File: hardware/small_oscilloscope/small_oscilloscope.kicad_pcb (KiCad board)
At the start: 2 copper layers, 181.6 x 99.1 mm, 104 parts, among them J1 Conn_01x16, J2 Conn_01x16, J3 Conn_Coaxial, J4 Conn_Coaxial, J5 Parellel LCD, J6 Conn_01x02, J7 Conn_01x03, Q1 NTR5103NT1G, Q2 NTR5103NT1G, Q3 NTR5103NT1G, Q4 NTR5103NT1G, Q5 NTR5103NT1G, Q6 NTR5103NT1G, Q7 NTR5103NT1G, Q8 NTR5103NT1G, Q9 NTR5103NT1G, SW1 SW_MEC_5E, SW2 RotaryEncoder_Switch_MP, SW3 SW_MEC_5E, SW4 SW_MEC_5E, SW5 SW_MEC_5E, SW6 RotaryEncoder_Switch_MP, U1 CH423S, U10 EA2208T6R, U11 FT800Q-T, U12 LM358, U13 L79L05_TO92, U2 TMUX1101DBV, U3 TMUX1101DBV, U4 TMUX1101DBV, U5 TMUX1101DBV, U6 TL084, U7 LM311, U8 LM311, U9 NE555P, Y1 12.0000M

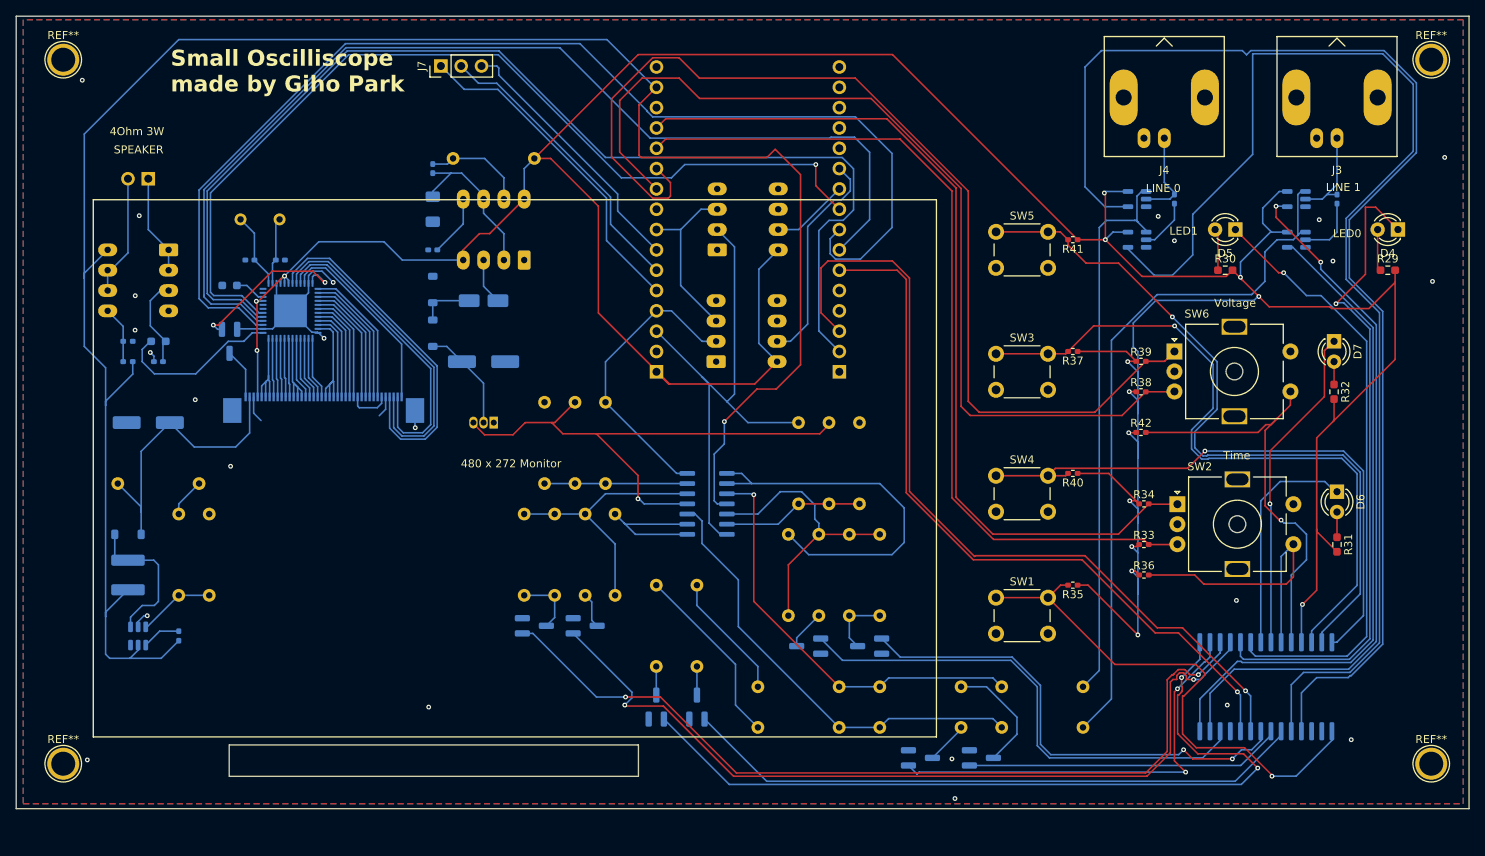
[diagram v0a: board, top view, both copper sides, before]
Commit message: oscilliscope first success
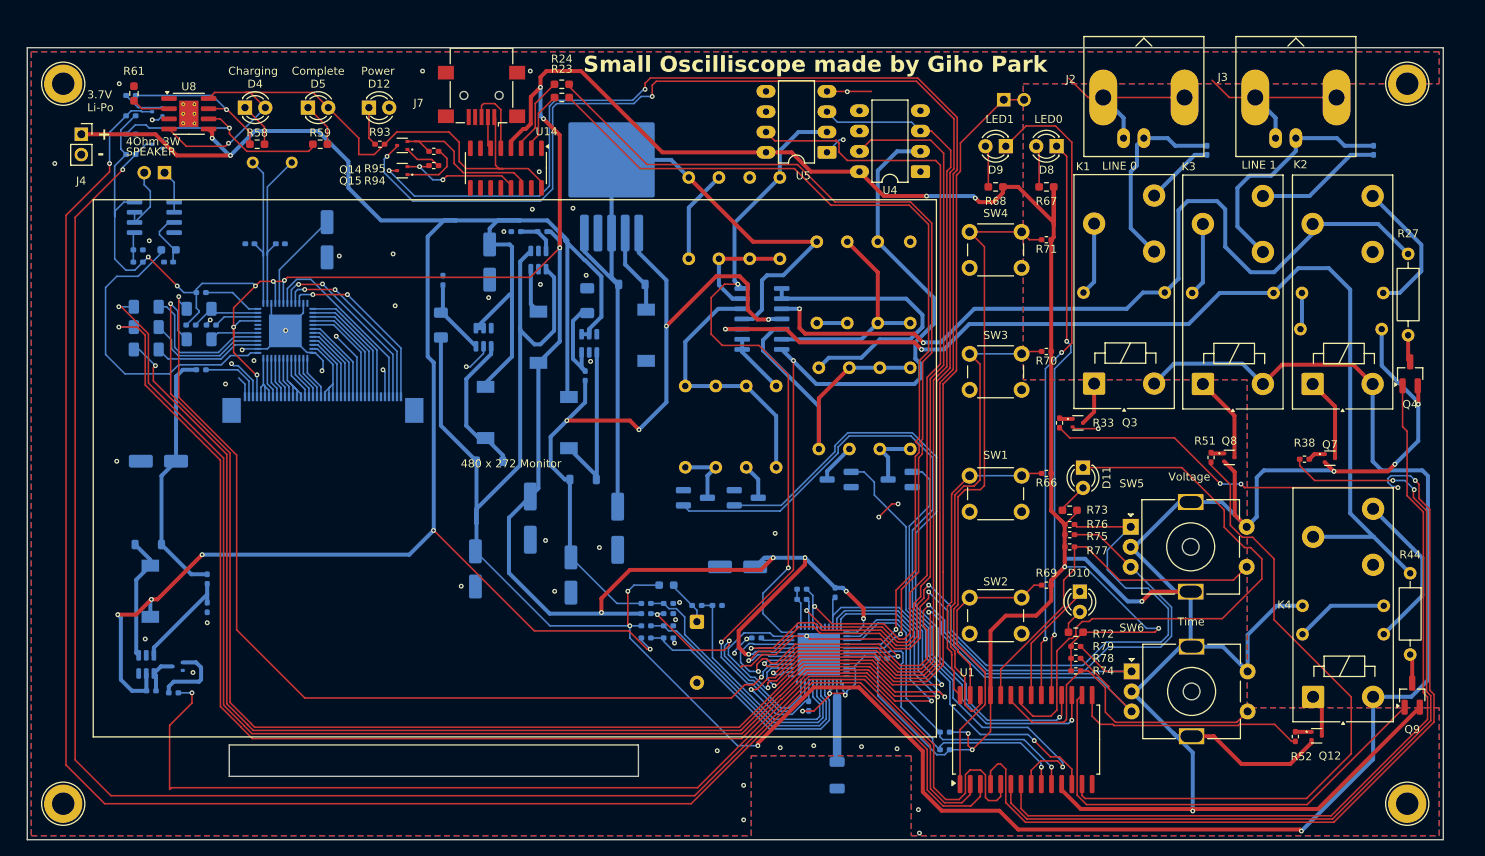
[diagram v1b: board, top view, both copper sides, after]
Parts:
- removed the C3 at (123.2, 59.7)
- removed the C4 at (123.2, 64.8)
- removed the C6 at (129.5, 78.7)
- removed the D2 at (123.2, 75.2)
- removed the J2 at (174.0, 80.0)
- removed the Q9 at (97.8, 76.2)
- removed the R25 at (123.2, 54.6)
- removed the R27 at (91.4, 97.8)
- removed the REF** at (248.0, 41.0)
- removed the REF** at (77.0, 41.0)
- removed the REF** at (77.0, 129.0)
- removed the REF** at (248.0, 129.0)
- removed the U13 at (130.8, 86.4)
- removed the U3 at (231.1, 58.4)
- removed the U4 at (211.2, 63.5)
- removed the U5 at (211.2, 58.4)
- added AE1: Antenna_Chip, Inductor_SMD:L_1206_3216Metric_Pad1.22x1.90mm_HandSolder, B.Cu at (173.7, 130.4)
- added C1: 10u, Capacitor_SMD:CP_Elec_5x5.3, B.Cu at (161.3, 104.4)
- added C10: 10u, Capacitor_SMD:CP_Elec_6.3x5.7, B.Cu at (146.3, 99.6)
- added C13: 10u, Capacitor_SMD:CP_Elec_5x5.3, B.Cu at (110.0, 63.5)
- added C2: 0.1u, Capacitor_SMD:C_0402_1005Metric_Pad0.74x0.62mm_HandSolder, B.Cu at (179.4, 115.8)
- added C7: 47u, Capacitor_SMD:CP_Elec_5x5.3, B.Cu at (140.5, 105.4)
- added C8: 100u, Capacitor_SMD:CP_Elec_5x5.3, B.Cu at (128.5, 104.6)
- added C9: 47u, Capacitor_SMD:CP_Elec_6.3x5.7, B.Cu at (135.4, 98.3)
- added D12: LED, LED_THT:LED_D3.0mm, F.Cu at (115.2, 47.0)
- added D3: 1N5819, Diode_SMD:D_SOD-123, B.Cu at (142.0, 93.5)
- added D4: LED_Small, LED_THT:LED_D3.0mm, F.Cu at (99.7, 47.0)
- added D5: LED_Small, LED_THT:LED_D3.0mm, F.Cu at (107.6, 47.0)
- added D6: 1N5819, Diode_SMD:D_SOD-123, B.Cu at (130.3, 91.2)
- added D7: 1N5819, Diode_SMD:D_SOD-123, B.Cu at (148.1, 69.1)
- added J4: BAT, Connector_PinSocket_2.54mm:PinSocket_1x02_P2.54mm_Vertical, F.Cu at (79.3, 50.3)
- added K1: FINDER-40.41, Relay_THT:Relay_SPDT_Finder_40.41, F.Cu at (205.9, 81.5)
- added K2: FINDER-40.41, Relay_THT:Relay_SPDT_Finder_40.41, F.Cu at (233.2, 81.5)
- added K3: FINDER-40.41, Relay_THT:Relay_SPDT_Finder_40.41, F.Cu at (219.5, 81.5)
- added K4: FINDER-40.41, Relay_THT:Relay_SPDT_Finder_40.41, F.Cu at (233.2, 120.6)
- added L2: 10u, Inductor_SMD:L_7.3x7.3_H3.5, B.Cu at (140.2, 86.4)
- added L3: 10u, Inductor_SMD:L_7.3x7.3_H3.5, B.Cu at (129.8, 85.1)
- added L4: 10u, Inductor_SMD:L_7.3x7.3_H3.5, B.Cu at (136.4, 75.7)
- added L5: 100u, Inductor_SMD:L_7.3x7.3_H3.5, B.Cu at (149.9, 75.4)
- added Q1: 2SC4671, Package_TO_SOT_SMD:SOT-523, B.Cu at (88.8, 47.5)
- added Q12: 2SC4671, Package_TO_SOT_SMD:SOT-523, F.Cu at (233.7, 125.5)
- added Q13: 2SC4671, Package_TO_SOT_SMD:SOT-523, B.Cu at (91.3, 116.8)
- added Q14: 2SC4671, Package_TO_SOT_SMD:SOT-523, F.Cu at (119.4, 51.7)
- added Q15: 2SC4671, Package_TO_SOT_SMD:SOT-523, F.Cu at (119.4, 54.9)
- added Q7: 2SC4671, Package_TO_SOT_SMD:SOT-523, F.Cu at (235.3, 90.8)
- added Q8: 2SC4671, Package_TO_SOT_SMD:SOT-523, F.Cu at (222.8, 90.7)
- added R10: 10k, Resistor_SMD:R_0402_1005Metric_Pad0.72x0.64mm_HandSolder, B.Cu at (85.5, 45.5)
- added R11: 10k, Resistor_SMD:R_0402_1005Metric_Pad0.72x0.64mm_HandSolder, B.Cu at (85.5, 50.3)
- added R12: 10K, Resistor_SMD:R_0402_1005Metric_Pad0.72x0.64mm_HandSolder, B.Cu at (156.2, 109.2)
- added R13: 100, Resistor_SMD:R_0603_1608Metric_Pad0.98x0.95mm_HandSolder, B.Cu at (152.4, 106.7)
- added R14: 10K, Resistor_SMD:R_0402_1005Metric_Pad0.72x0.64mm_HandSolder, B.Cu at (149.9, 113.3)
- added R15: 10K, Resistor_SMD:R_0402_1005Metric_Pad0.72x0.64mm_HandSolder, B.Cu at (149.9, 111.8)
- added R16: 4K7, Resistor_SMD:R_0402_1005Metric_Pad0.72x0.64mm_HandSolder, B.Cu at (149.9, 109.0)
- added R17: 10K, Resistor_SMD:R_0402_1005Metric_Pad0.72x0.64mm_HandSolder, B.Cu at (149.9, 110.2)
- added R18: 10K, Resistor_SMD:R_0402_1005Metric_Pad0.72x0.64mm_HandSolder, B.Cu at (152.7, 113.3)
- added R19: 3K, Resistor_SMD:R_0402_1005Metric_Pad0.72x0.64mm_HandSolder, B.Cu at (152.7, 111.8)
- added R2: 10k, Resistor_SMD:R_0402_1005Metric_Pad0.72x0.64mm_HandSolder, B.Cu at (187.2, 125.1)
- added R20: 820R, Resistor_SMD:R_0402_1005Metric_Pad0.72x0.64mm_HandSolder, B.Cu at (152.7, 109.0)
- added R22: 10K, Resistor_SMD:R_0402_1005Metric_Pad0.72x0.64mm_HandSolder, B.Cu at (158.8, 109.2)
- added R23: 1k, Resistor_SMD:R_0603_1608Metric_Pad0.98x0.95mm_HandSolder, F.Cu at (139.3, 45.7)
- added R3: 10k, Resistor_SMD:R_0402_1005Metric_Pad0.72x0.64mm_HandSolder, B.Cu at (170.2, 121.8)
- added R33: 3k, Resistor_SMD:R_0402_1005Metric_Pad0.72x0.64mm_HandSolder, F.Cu at (201.5, 86.4)
- added R35: 3K6, Resistor_THT:R_Axial_DIN0207_L6.3mm_D2.5mm_P10.16mm_Horizontal, B.Cu at (175.0, 63.8)
- added R38: 3k, Resistor_SMD:R_0402_1005Metric_Pad0.72x0.64mm_HandSolder, F.Cu at (232.2, 90.9)
- added R4: 10k, Resistor_SMD:R_0402_1005Metric_Pad0.72x0.64mm_HandSolder, B.Cu at (163.7, 113.3)
- added R42: 3K6, Resistor_THT:R_Axial_DIN0207_L6.3mm_D2.5mm_P10.16mm_Horizontal, B.Cu at (159.0, 65.9)
- added R43: 3K6, Resistor_THT:R_Axial_DIN0207_L6.3mm_D2.5mm_P10.16mm_Horizontal, B.Cu at (155.2, 65.9)
- added R5: 10k, Resistor_SMD:R_0402_1005Metric_Pad0.72x0.64mm_HandSolder, B.Cu at (169.3, 107.2)
- added R51: 3k, Resistor_SMD:R_0402_1005Metric_Pad0.72x0.64mm_HandSolder, F.Cu at (220.5, 90.7)
- added R52: 3k, Resistor_SMD:R_0402_1005Metric_Pad0.72x0.64mm_HandSolder, F.Cu at (231.0, 125.6)
- added R54: 10k, Resistor_SMD:R_0402_1005Metric_Pad0.72x0.64mm_HandSolder, B.Cu at (88.0, 119.9)
- added R56: 10k, Resistor_SMD:R_0402_1005Metric_Pad0.72x0.64mm_HandSolder, B.Cu at (90.8, 120.1)
- added R57: 147k, Resistor_SMD:R_0402_1005Metric_Pad0.72x0.64mm_HandSolder, B.Cu at (142.2, 80.5)
- added R58: 1k, Resistor_SMD:R_0603_1608Metric_Pad0.98x0.95mm_HandSolder, F.Cu at (101.2, 51.6)
- added R59: 1k, Resistor_SMD:R_0603_1608Metric_Pad0.98x0.95mm_HandSolder, F.Cu at (109.1, 51.6)
- added R6: 10k, Resistor_SMD:R_0402_1005Metric_Pad0.72x0.64mm_HandSolder, B.Cu at (169.3, 108.5)
- added R60: 7.5k, Resistor_SMD:R_1206_3216Metric_Pad1.30x1.75mm_HandSolder, B.Cu at (142.5, 71.1)
- added R61: 1k, Resistor_SMD:R_0603_1608Metric_Pad0.98x0.95mm_HandSolder, F.Cu at (85.8, 45.2)
- added R62: 22k, Resistor_SMD:R_1206_3216Metric_Pad1.30x1.75mm_HandSolder, B.Cu at (124.2, 74.2)
- added R63: 470k, Resistor_SMD:R_0402_1005Metric_Pad0.72x0.64mm_HandSolder, B.Cu at (136.9, 62.5)
- added R64: 3k, Resistor_SMD:R_0402_1005Metric_Pad0.72x0.64mm_HandSolder, B.Cu at (124.5, 68.6)
- added R65: 100k, Resistor_SMD:R_0402_1005Metric_Pad0.72x0.64mm_HandSolder, B.Cu at (133.6, 62.5)
- added R7: 10k, Resistor_SMD:R_0402_1005Metric_Pad0.72x0.64mm_HandSolder, B.Cu at (173.5, 107.6)
- added R8: 10k, Resistor_SMD:R_0402_1005Metric_Pad0.72x0.64mm_HandSolder, B.Cu at (85.5, 48.0)
- added R80: 150, Resistor_SMD:R_0402_1005Metric_Pad0.72x0.64mm_HandSolder, B.Cu at (94.2, 79.8)
- added R81: 10k, Resistor_SMD:R_0402_1005Metric_Pad0.72x0.64mm_HandSolder, B.Cu at (93.0, 74.2)
- added R82: 10k, Resistor_SMD:R_0402_1005Metric_Pad0.72x0.64mm_HandSolder, B.Cu at (94.2, 70.1)
- added R83: 10R, Resistor_SMD:R_1206_3216Metric_Pad1.30x1.75mm_HandSolder, B.Cu at (87.4, 77.2)
- added R84: 10R, Resistor_SMD:R_1206_3216Metric_Pad1.30x1.75mm_HandSolder, B.Cu at (87.4, 74.4)
- added R85: 10R, Resistor_SMD:R_1206_3216Metric_Pad1.30x1.75mm_HandSolder, B.Cu at (87.4, 71.9)
- added R86: 10R, Resistor_SMD:R_1206_3216Metric_Pad1.30x1.75mm_HandSolder, B.Cu at (94.0, 75.9)
- added R87: 10R, Resistor_SMD:R_1206_3216Metric_Pad1.30x1.75mm_HandSolder, B.Cu at (94.0, 72.1)
- added R9: 10k, Resistor_SMD:R_0402_1005Metric_Pad0.72x0.64mm_HandSolder, B.Cu at (85.5, 52.8)
- added R93: 3k, Resistor_SMD:R_0402_1005Metric_Pad0.72x0.64mm_HandSolder, F.Cu at (116.6, 51.6)
- added R94: 10k, Resistor_SMD:R_0402_1005Metric_Pad0.72x0.64mm_HandSolder, F.Cu at (123.3, 54.2)
- added R95: 10k, Resistor_SMD:R_0402_1005Metric_Pad0.72x0.64mm_HandSolder, F.Cu at (123.3, 52.5)
- added REF**: TestPoint_Loop_D3.80mm_Drill2.8mm, TestPoint:TestPoint_Loop_D3.80mm_Drill2.8mm, F.Cu at (245.0, 44.0)
- added REF**: TestPoint_Loop_D3.80mm_Drill2.8mm, TestPoint:TestPoint_Loop_D3.80mm_Drill2.8mm, F.Cu at (245.0, 134.0)
- added REF**: TestPoint_Loop_D3.80mm_Drill2.8mm, TestPoint:TestPoint_Loop_D3.80mm_Drill2.8mm, F.Cu at (77.0, 134.0)
- added REF**: TestPoint_Loop_D3.80mm_Drill2.8mm, TestPoint:TestPoint_Loop_D3.80mm_Drill2.8mm, F.Cu at (77.0, 44.0)
- added U10: EA8105, Package_TO_SOT_SMD:SOT-23-6, B.Cu at (136.4, 66.0)
- added U11: LM2576S-12, Package_TO_SOT_SMD:TO-263-5_TabPin3, B.Cu at (145.5, 55.0)
- added U14: CH340C, Package_SO:SOIC-16_3.9x9.9mm_P1.27mm, F.Cu at (132.3, 54.5)
- added U7: EA2208T6R, Package_TO_SOT_SMD:SOT-23-6, B.Cu at (142.7, 76.5)
- added U8: TP4056-42-ESOP8, Package_SO:SOIC-8-1EP_3.9x4.9mm_P1.27mm_EP2.41x3.3mm_ThermalVias, F.Cu at (92.7, 47.8)
- C5: value 10u -> 100u; footprint Capacitor_SMD:CP_Elec_4x5.7 -> Capacitor_SMD:CP_Elec_5x5.3
- C6: renamed from C7; value 47u -> 10u; footprint Capacitor_SMD:CP_Elec_6.3x5.7 -> Capacitor_SMD:CP_Elec_5x5.3
- D1: value D_Schottky -> 1N5225B; footprint Diode_SMD:D_SOD-123 -> Diode_THT:D_A-405_P7.62mm_Horizontal
- J1: value Conn_01x16 -> SIGNAL; footprint Connector_PinSocket_2.54mm:PinSocket_1x16_P2.54mm_Vertical -> Connector_PinSocket_2.54mm:PinSocket_1x02_P2.54mm_Vertical
- J6: value Conn_01x02 -> SPEAKER; footprint Connector_PinHeader_2.54mm:PinHeader_1x02_P2.54mm_Vertical -> Connector_PinSocket_2.54mm:PinSocket_1x02_P2.54mm_Vertical
- J7: value Conn_01x03 -> USB_B_Mini; footprint Connector_PinHeader_2.54mm:PinHeader_1x03_P2.54mm_Vertical -> Connector_USB:USB_Mini-B_Lumberg_2486_01_Horizontal
- L1: value 1u -> 10u; footprint Inductor_SMD:L_Changjiang_FNR5045S -> Inductor_SMD:L_7.3x7.3_H3.5
- Q10: renamed from Q5; value NTR5103NT1G -> BSS138
- Q11: renamed from Q7; value NTR5103NT1G -> BSS138
- Q2: value NTR5103NT1G -> 2SC4671; footprint Package_TO_SOT_SMD:SOT-23_Handsoldering -> Package_TO_SOT_SMD:SOT-523
- Q3: value NTR5103NT1G -> 2SC4671; footprint Package_TO_SOT_SMD:SOT-23_Handsoldering -> Package_TO_SOT_SMD:SOT-523; moved to F.Cu
- Q4: value NTR5103NT1G -> BSS138; moved to F.Cu
- Q5: renamed from Q6; value NTR5103NT1G -> BSS138
- Q6: renamed from Q8; value NTR5103NT1G -> BSS138
- Q9: renamed from Q1; value NTR5103NT1G -> BSS138; moved to F.Cu
- R21: value 3K -> 10K; footprint Resistor_THT:R_Axial_DIN0207_L6.3mm_D2.5mm_P10.16mm_Horizontal -> Resistor_SMD:R_0402_1005Metric_Pad0.72x0.64mm_HandSolder
- R24: value 560 -> 1k; footprint Resistor_THT:R_Axial_DIN0207_L6.3mm_D2.5mm_P10.16mm_Horizontal -> Resistor_SMD:R_0603_1608Metric_Pad0.98x0.95mm_HandSolder; moved to F.Cu
- R27: renamed from R5; moved to F.Cu
- R30: renamed from R15; value 500 -> 500R
- R31: renamed from R17; value 500 -> 500R
- R36: renamed from R23; value 3K -> 3K6
- R37: renamed from R19; value 150 -> 150R
- R44: renamed from R3; moved to F.Cu
- R47: renamed from R14; value 500 -> 500R
- R48: renamed from R16; value 500 -> 500R
- R49: renamed from R18; value 150 -> 150R
- R53: renamed from R26; value 10k -> 4.7k; footprint Resistor_THT:R_Axial_DIN0207_L6.3mm_D2.5mm_P10.16mm_Horizontal -> Resistor_SMD:R_0402_1005Metric_Pad0.72x0.64mm_HandSolder
- R55: renamed from R28; value 500 -> 120; footprint Resistor_THT:R_Axial_DIN0207_L6.3mm_D2.5mm_P10.16mm_Horizontal -> Resistor_SMD:R_0402_1005Metric_Pad0.72x0.64mm_HandSolder
- R89: renamed from R43; value 1k -> 10k; footprint Resistor_SMD:R_0603_1608Metric_Pad0.98x0.95mm_HandSolder -> Resistor_SMD:R_0402_1005Metric_Pad0.72x0.64mm_HandSolder
- U1: moved to F.Cu
- U13: renamed from U12; footprint Package_DIP:DIP-8_W7.62mm_LongPads -> Package_SO:SOIC-8_3.9x4.9mm_P1.27mm
- U2: value TMUX1101DBV -> ESP32-PICO-D4; footprint Package_TO_SOT_SMD:SOT-23-5 -> Package_DFN_QFN:QFN-48-1EP_7x7mm_P0.5mm_EP5.3x5.3mm
- U4: renamed from U7; moved to F.Cu
- U5: renamed from U8; moved to F.Cu
- U9: value NE555P -> EA2208T6R; footprint Package_DIP:DIP-8_W7.62mm_LongPads -> Package_TO_SOT_SMD:SOT-23-6
- moved Q2 128.4 mm to (88.8, 51.6), turned to 180 degrees
- moved Q4 98.4 mm to (245.4, 80.3)
- moved R1 96.8 mm to (187.2, 127.3), turned to 180 degrees
- moved R50 91.0 mm to (242.1, 109.3), turned to 180 degrees
- moved R27 85.4 mm to (245.1, 65.3), turned to -90 degrees
- moved R28 84.0 mm to (242.0, 70.2)
- moved R32 81.9 mm to (231.6, 74.7), turned to 0 degrees
- moved U2 79.0 mm to (171.4, 115.3), turned to 90 degrees
- moved R45 69.1 mm to (242.1, 112.8)
- moved R44 69.0 mm to (245.4, 105.2), turned to -90 degrees
- moved Q3 63.5 mm to (203.8, 86.4), turned to 0 degrees
- moved Q9 62.0 mm to (245.6, 120.4), turned to 90 degrees
- moved R39 56.0 mm to (218.1, 70.2), turned to 0 degrees
- moved J1 55.1 mm to (194.6, 46.0), turned to -90 degrees
- moved D1 53.1 mm to (156.2, 111.3)
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- renumbered C8 to C11, C9 to C12, C10 to C14, C2 to C3, C1 to C4, D6 to D10, D7 to D11, D3 to D2, D4 to D8, D5 to D9, J4 to J2, R4 to R25, R12 to R26, R8 to R28, R13 to R29, R9 to R32, R22 to R34, R2 to R39, R10 to R40, R20 to R41, R6 to R45, R11 to R46, R7 to R50, R40 to R66, R29 to R67, R30 to R68, R35 to R69, R37 to R70, R41 to R71, R31 to R72, R32 to R73, R36 to R74, R38 to R75, R39 to R76, R42 to R77, R33 to R78, R34 to R79, R44 to R90, R45 to R91, R46 to R92, SW4 to SW1, SW1 to SW2, SW5 to SW4, SW6 to SW5, SW2 to SW6, U11 to U12, U6 to U3, U10 to U6
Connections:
- C4 pad 2: Net-(C1-Pad2) -> Net-(C4-Pad2)
- C5 pad 1: Net-(U9-Q) -> Vbat
- C5 pad 2: Net-(D1-A) -> GND
- D1 pad 1: GND -> Net-(D1-K)
- D1 pad 2: Net-(D1-A) -> GND
- J1 pad 1: +3.3V -> /TESTPIN
- J1 pad 2: unconnected-(J1-RESET-Pad2) -> /TESTPIN
- J5 pad 39: +24V -> Net-(J5-LEDA)
- J5 pad 40: Net-(J5-LEDK) -> GND
- J5 pad 6: GND -> unconnected-(J5-NC-Pad6)
- J7 pad 1: Net-(J1-34) -> Vusb
- J7 pad 2: Net-(J1-32) -> Net-(J7-D-)
- J7 pad 3: Net-(J1-33) -> Net-(J7-D+)
- L1 pad 1: +5V -> Vbat
- Q2 pad 1: /Q4 -> Net-(Q2-B)
- Q2 pad 3: Net-(Q2-D) -> /~{STDBY}
- Q3 pad 1: /Q9 -> Net-(Q3-B)
- Q3 pad 3: Net-(Q3-D) -> Net-(Q3-C)
- Q4 pad 1: /Q3 -> /Q4
- R1 pad 1: +5V -> +3.3V
- R1 pad 2: /Power/BACKLIGHT -> /SCL
- R21 pad 1: Net-(U6D--) -> /VREF3V3
- R21 pad 2: -5V -> GND
- R24 pad 1: +3.3V -> /USB Serial/RXD
- R24 pad 2: Net-(U9-DIS) -> /TXD
- R25 pad 2: Net-(U6A-+) -> Net-(U3A-+)
- R27 pad 1: Net-(U6A-+) -> Net-(U3A-+)
- R27 pad 2: Net-(Q2-D) -> Net-(Q4-D)
- R28 pad 1: Net-(U6A-+) -> Net-(K2-Pad14)
- R32 pad 2: Net-(Q4-D) -> GND
- R34 pad 1: Net-(U6B--) -> Net-(U3B--)
- R36 pad 1: Net-(U6B--) -> Net-(R35-Pad2)
- R36 pad 2: -5V -> -12V
- R37 pad 1: Net-(U6B--) -> Net-(U3B--)
- R39 pad 1: Net-(R2-Pad1) -> Net-(K3-Pad11)
- R39 pad 2: Net-(U6C-+) -> Net-(U3C-+)
- R41 pad 1: Net-(U6D--) -> Net-(U3D--)
- R44 pad 1: Net-(U6C-+) -> Net-(U3C-+)
- R45 pad 1: Net-(U6C-+) -> Net-(K4-Pad14)
- R49 pad 1: Net-(U6D--) -> Net-(U3D--)
- R50 pad 2: Net-(Q3-D) -> GND
- R53 pad 2: Net-(R26-Pad2) -> Net-(U6-FB)
- R55 pad 1: Net-(U10-FB) -> Net-(U6-FB)
- R91 pad 1: +5V -> +3.3V
- U1 pad 14: /Q8 -> unconnected-(U1-OC7-Pad14)
- U1 pad 2: unconnected-(U1-IO6-Pad2) -> /~{STDBY}
- U1 pad 3: unconnected-(U1-IO7-Pad3) -> /~{CHRG}
- U1 pad 5: /Q2 -> /BACKLIGHT
- U12 pad 11: unconnected-(U11-INT_N-Pad11) -> Net-(U12-INT_N)
- U12 pad 12: unconnected-(U11-PD_N-Pad12) -> Net-(U12-PD_N)
- U12 pad 17: +3.3V -> Net-(U12-VCC1V2)
- U12 pad 24: Net-(Q9-G) -> unconnected-(U12-BACKLIGHT-Pad24)
- U12 pad 3: /SCK -> Net-(U12-SPI_SCLK/_I2C_SCL)
- U12 pad 4: /MISO -> Net-(U12-MISO/_I2C_SDA)
- U12 pad 5: /MOSI -> Net-(U12-MOSI/_I2C_SA0)
- U12 pad 6: /SS -> Net-(U12-CS_N/_I2C_SA1)
- U13 pad 8: +5V -> +3.3V
- U2 pad 1: Net-(R2-Pad1) -> +3.3V
- U2 pad 2: Net-(C1-Pad2) -> /ANT50R
- U2 pad 3: GND -> +3.3V
- U2 pad 4: /Q8 -> +3.3V
- U2 pad 5: +3.3V -> /VREFBAT
- U3 pad 10: Net-(U6C-+) -> Net-(U3C-+)
- U3 pad 11: -5V -> -12V
- U3 pad 13: Net-(U6D--) -> Net-(U3D--)
- U3 pad 3: Net-(U6A-+) -> Net-(U3A-+)
- U3 pad 4: +5V -> +12V
- U3 pad 6: Net-(U6B--) -> Net-(U3B--)
- U6 pad 3: Net-(U10-FB) -> Net-(U6-FB)
- U6 pad 4: /Power/BACKLIGHT -> Net-(Q13-C)
- U6 pad 5: +5V -> Vbat
- U9 pad 1: GND -> Net-(D6-A)
- U9 pad 2: Net-(U9-THR) -> GND
- U9 pad 3: Net-(U9-Q) -> Net-(U9-FB)
- U9 pad 4: +3.3V -> Vbat
- U9 pad 5: Net-(U9-CV) -> Vbat
- U9 pad 6: Net-(U9-THR) -> unconnected-(U9-NC-Pad6)
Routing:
- net GND: track 43.5 -> 372.7 mm, vias 24 -> 62
- net Vbat: track 0.00 -> 283.2 mm, vias 0 -> 7
- net /~{CHRG}: track 0.00 -> 221.8 mm, vias 0 -> 1
- net /~{STDBY}: track 0.00 -> 212.4 mm, vias 0 -> 1
- net /EN: track 0.00 -> 199.3 mm, vias 0 -> 3
- net /IO0: track 0.00 -> 198.6 mm, vias 0 -> 3
- net /Q2: track 154.7 -> 0.00 mm
- net /BACKLIGHT: track 0.00 -> 142.1 mm, vias 0 -> 1
- net Net-(U3C-+): track 0.00 -> 132.0 mm, vias 0 -> 2
- net /~{INT}: track 0.00 -> 121.5 mm, vias 0 -> 2
- net /TXD: track 0.00 -> 113.4 mm, vias 0 -> 1
- net /RXD: track 0.00 -> 111.1 mm, vias 0 -> 1
- net /TESTPIN: track 0.00 -> 106.0 mm, vias 0 -> 1
- net Net-(U3A-+): track 0.00 -> 105.0 mm, vias 0 -> 2
- net -12V: track 0.00 -> 97.4 mm
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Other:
- board size 181.6 x 99.1 mm -> 177 x 99 mm
- board text added: "+ -"
- board text added: "3.7V Li-Po"
- board text added: "Charging"
- board text added: "Complete"
- board text added: "Power"
- board text removed: "LOLIN D32"
